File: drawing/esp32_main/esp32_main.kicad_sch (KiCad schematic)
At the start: 4 parts, among them U1_Master ESP32-WROOM-32, U2_Slave ESP32-WROOM-32, U3 MAX3485, U4 MAX3485

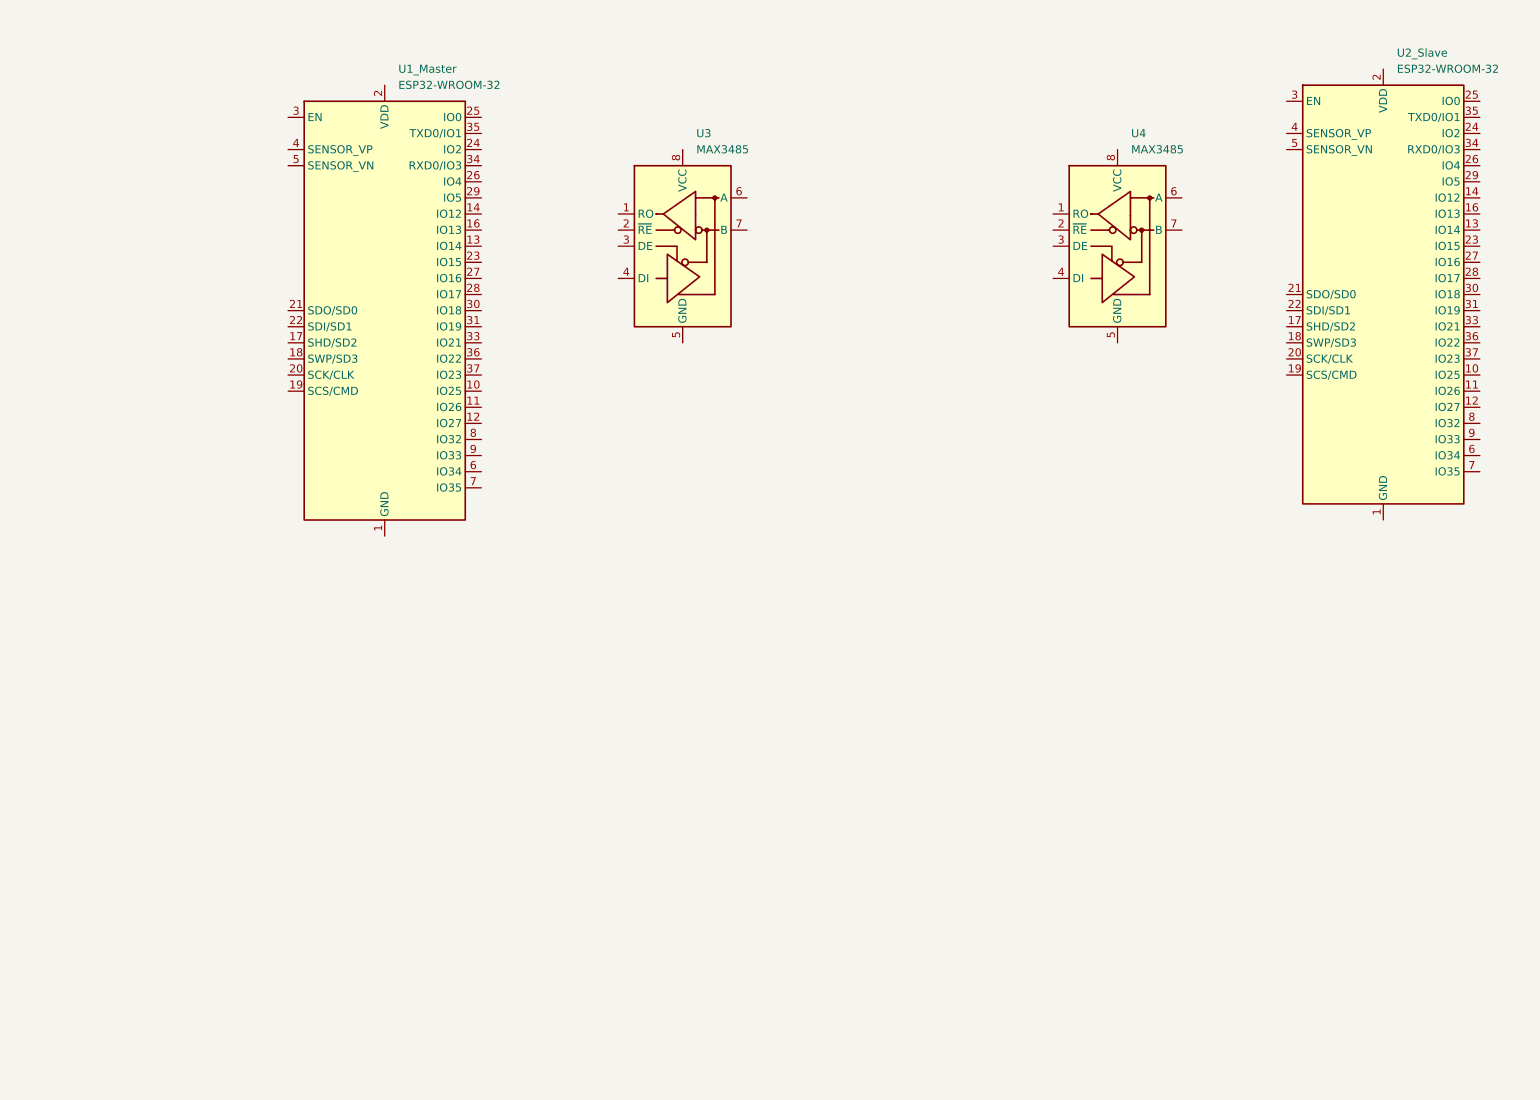
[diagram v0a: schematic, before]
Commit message: kicad update
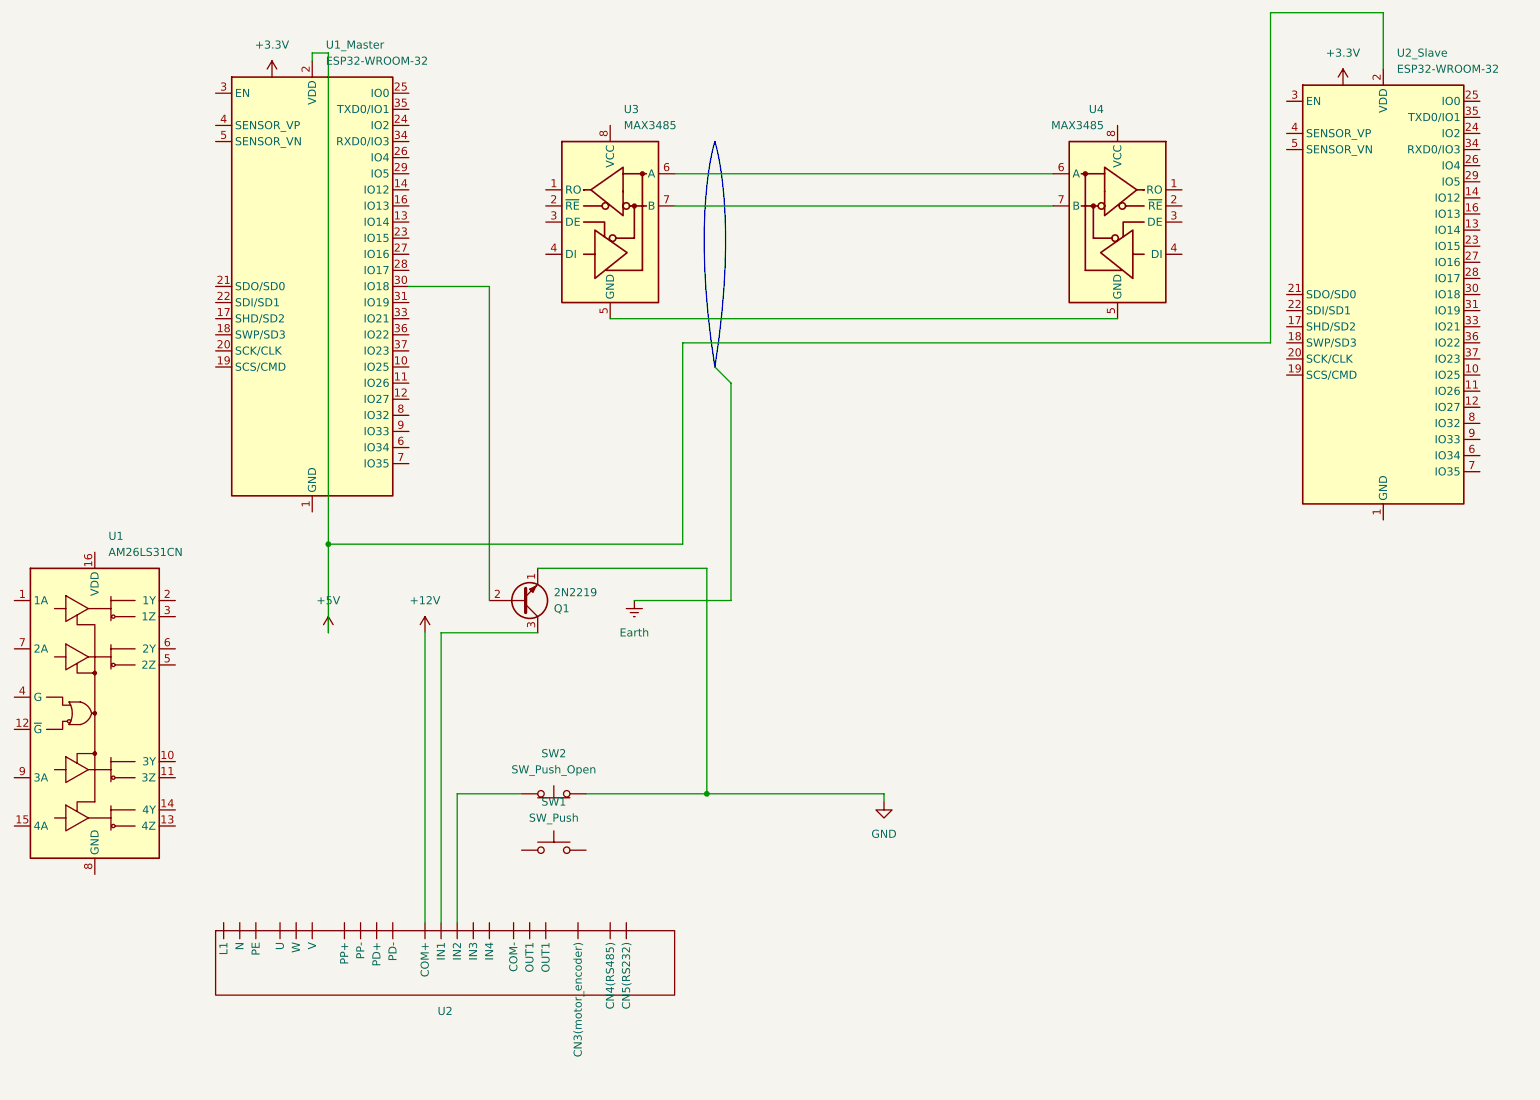
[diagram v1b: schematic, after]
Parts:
- added Q1: 2N2219, Package_TO_SOT_THT:TO-39-3, symbol Transistor_BJT:2N2219
- added SW1: SW_Push, symbol Switch:SW_Push
- added SW2: SW_Push_Open, symbol Switch:SW_Push_Open
- added U1: AM26LS31CN, Package_DIP:DIP-16_W7.62mm, symbol Interface:AM26LS31CN
- added U2: (no value), symbol GlasAutoma]:T6_Drive
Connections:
- net +5V: now reaches U2_Slave.2 (VDD)
- net +5V: now also U1_Master.2 (VDD)
- net at U3.5 (GND): now also U4.5 (GND)
- net at U3.6 (A): now also U4.6 (A)
- net at U3.7 (B): now also U4.7 (B)
- net at U1_Master.30 (IO18): now also Q1.2 (B)
- new net: SW2.1 (A), U2. (CN5(RS232))
- new net: Q1.3 (C), U2. (CN5(RS232))
- new net +12V: U2. (CN5(RS232))
- new net GND: Q1.1 (E), SW2.2 (B)
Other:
- moved on the sheet: U1_Master, U3, U4
